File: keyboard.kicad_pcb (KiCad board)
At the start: 2 copper layers, 168.3 x 124.5 mm, 135 parts, among them J1 Conn_01x06_Socket, J2 Conn_01x02_Socket, J3 Conn_01x02_Socket, J4 Conn_01x06_Socket, SW1 SW_Push, SW10 SW_Push, SW11 SW_Push, SW12 SW_Push, SW13 SW_Push, SW14 SW_Push, SW15 SW_Push, SW16 SW_Push, SW17 SW_Push, SW18 SW_Push, SW19 SW_Push, SW2 SW_Push, SW20 SW_Push, SW21 SW_Push, SW22 SW_Push, SW23 SW_Push, SW24 SW_Push, SW25 SW_Push, SW26 SW_Push, SW27 SW_Push, SW28 SW_Push, SW29 SW_Push, SW3 SW_Push, SW30 SW_Push, SW31 SW_Push, SW32 SW_Push, SW33 SW_Push, SW34 SW_Push, SW35 SW_Push, SW36 SW_Push, SW37 SW_Push, SW38 SW_Push, SW39 SW_Push, SW4 SW_Push, SW40 SW_Push, SW41 SW_Push, SW42 SW_Push, SW43 SW_Push, SW44 SW_Push, SW45 SW_Push, SW46 SW_Push, SW47 SW_Push, SW48 SW_Push, SW49 SW_Push, SW5 SW_Push, SW50 SW_Push, SW51 SW_Push, SW52 SW_Push, SW53 SW_Push, SW54 SW_Push, SW55 SW_Push, SW56 SW_Push, SW57 SW_Push, SW58 SW_Push, SW59 SW_Push, SW6 SW_Push, SW60 SW_Push, SW7 SW_Push, SW8 SW_Push, SW9 SW_Push, U1 rp2040-zero

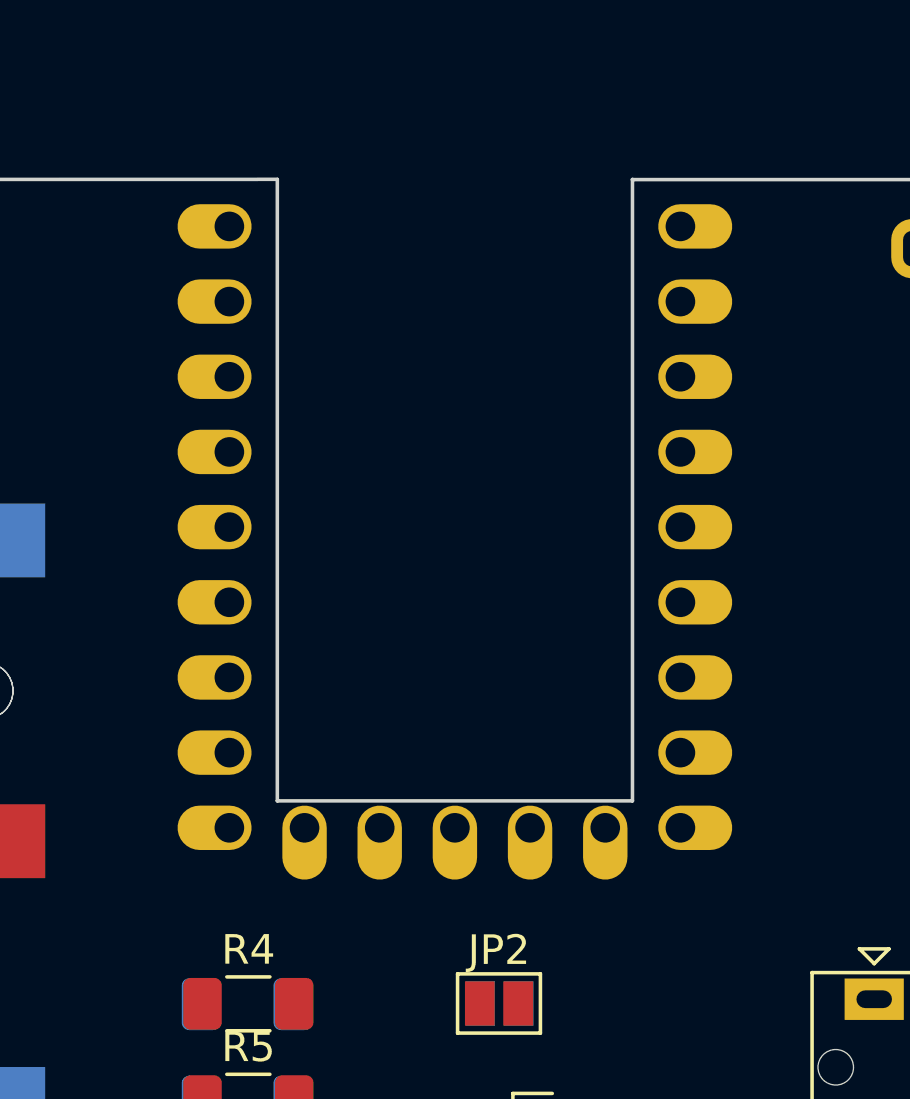
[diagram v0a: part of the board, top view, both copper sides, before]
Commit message: 実は耐えてた
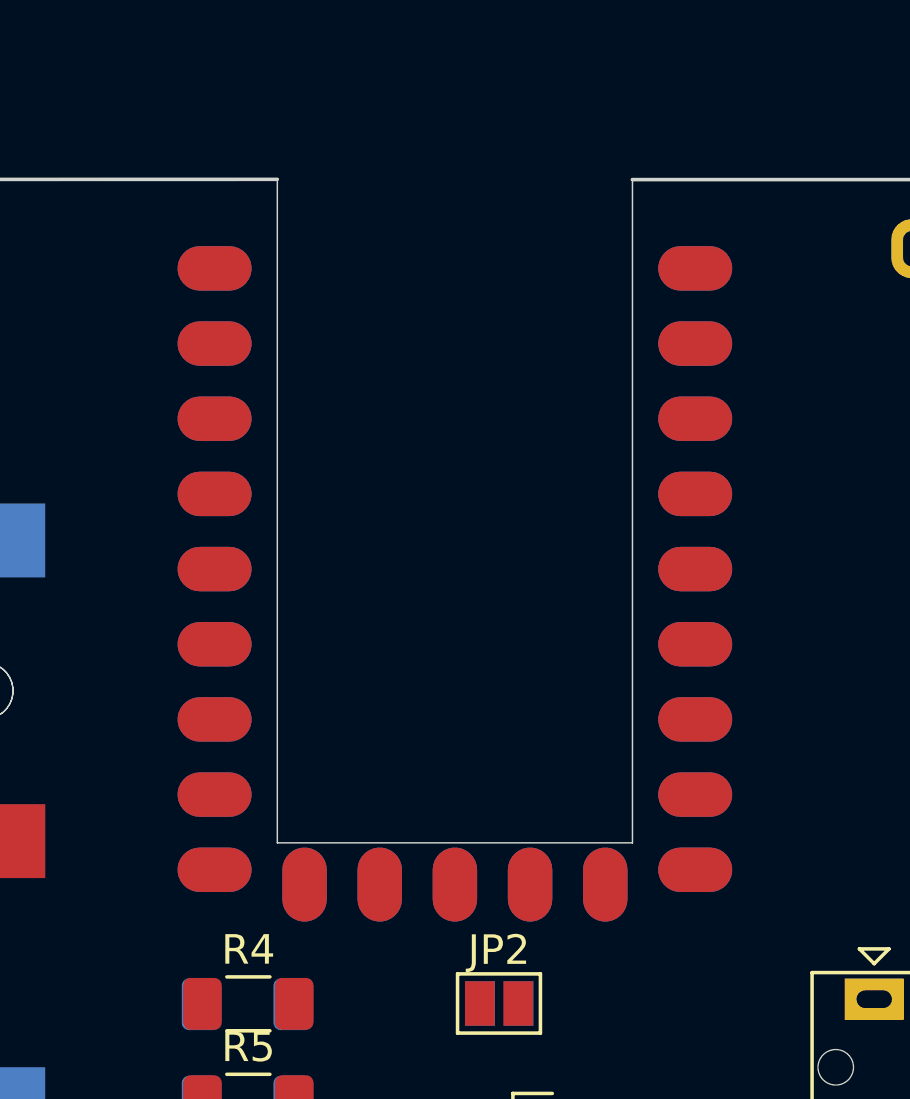
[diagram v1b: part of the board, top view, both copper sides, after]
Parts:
- added U2: rp2040-zero, mcu:rp2040-zero-smd_reverse_flush_B, B.Cu at (192.4, 55.6)
- U1: footprint mcu:rp2040-zero-tht -> mcu:rp2040-zero-smd_reverse_flush_A; moved to F.Cu
- moved U1 1.42 mm to (192.4, 55.6), turned to 0 degrees
